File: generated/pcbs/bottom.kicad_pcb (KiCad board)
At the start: 2 copper layers, 131.7 x 96.3 mm, 5 parts

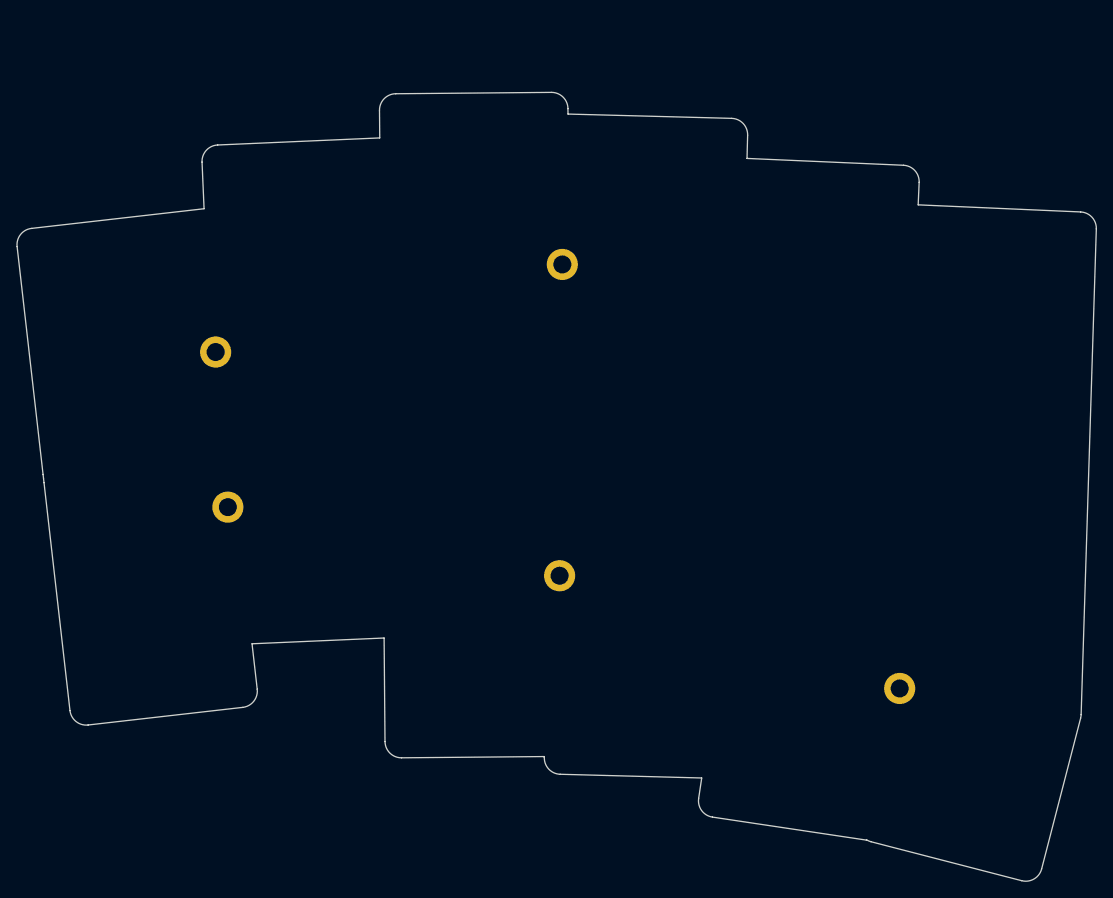
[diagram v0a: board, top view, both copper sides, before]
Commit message: Start messing around with choc
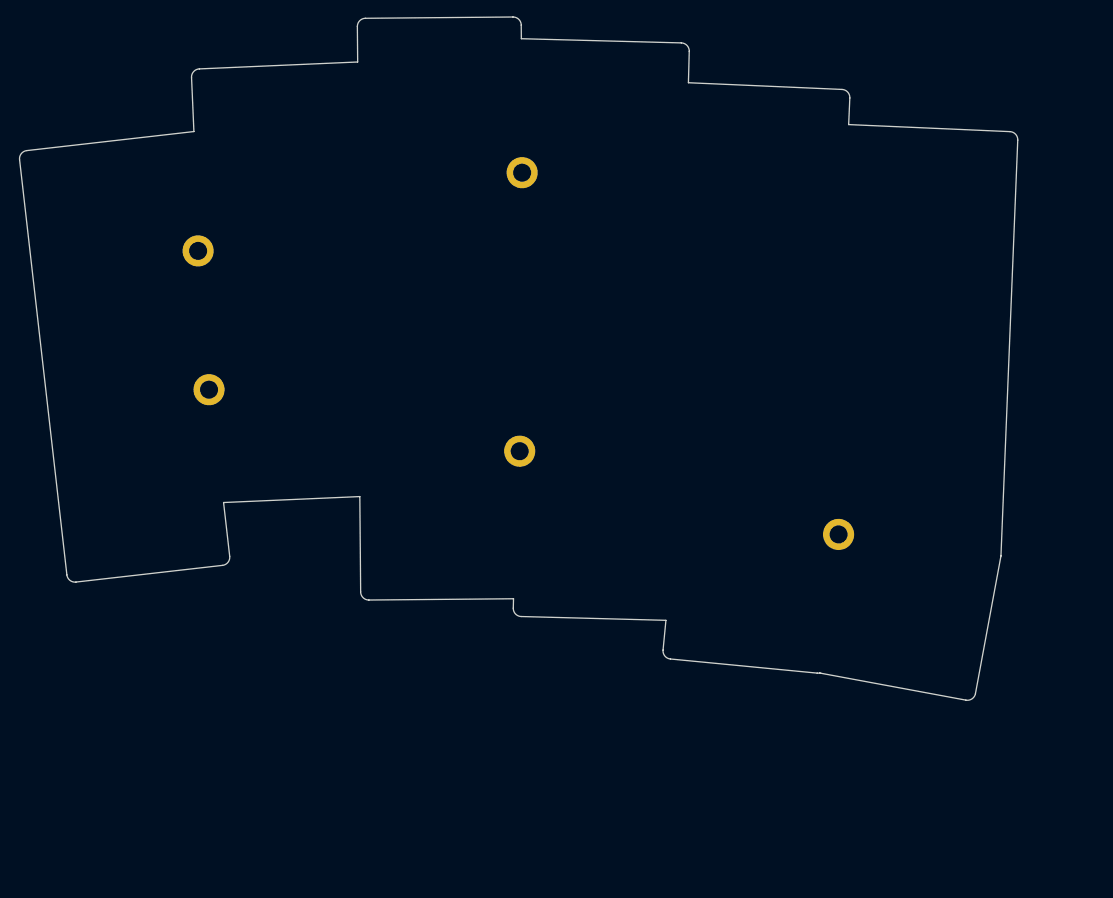
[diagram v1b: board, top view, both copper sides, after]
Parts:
- moved H5 20.2 mm to (263.3, 154.4), turned to -8 degrees
- moved H4 16.0 mm to (224.4, 144.3)
- moved H2 14.5 mm to (186.5, 136.8)
- moved H1 12.5 mm to (185.1, 119.8)
- moved H3 12.2 mm to (224.7, 110.3)
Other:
- board size 131.7 x 96.3 mm -> 121.8 x 83.4 mm
